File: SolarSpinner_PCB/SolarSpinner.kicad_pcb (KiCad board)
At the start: 2 copper layers, 50 x 40 mm, 21 parts, among them IC1 ATTINY85-P, P1 SOLAR, P10 HOLES, P2 SOLAR_V, P3 MOTOR, P4 ISP, P5 HEADER, P7 LOGO1, P8 LOGO2, Q1 Q_NPN_CBE

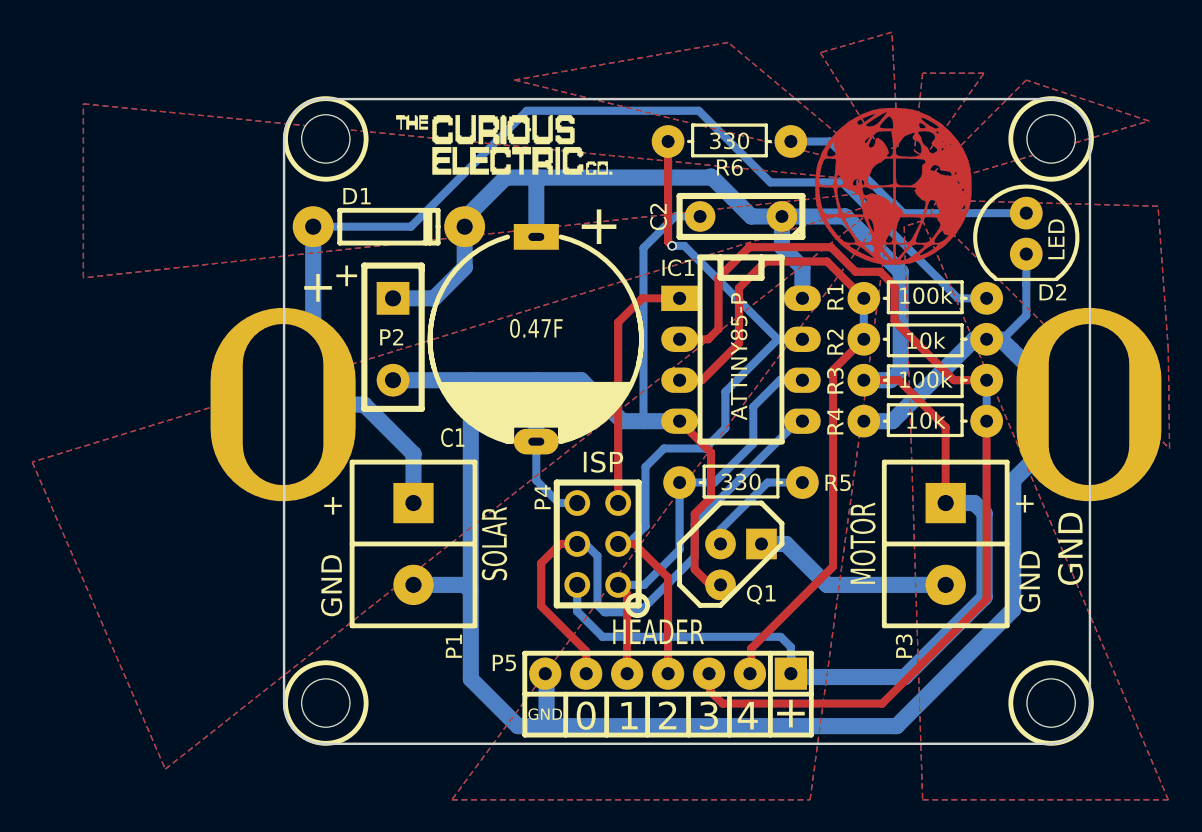
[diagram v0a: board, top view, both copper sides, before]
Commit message: Updated PCB. New Gerber
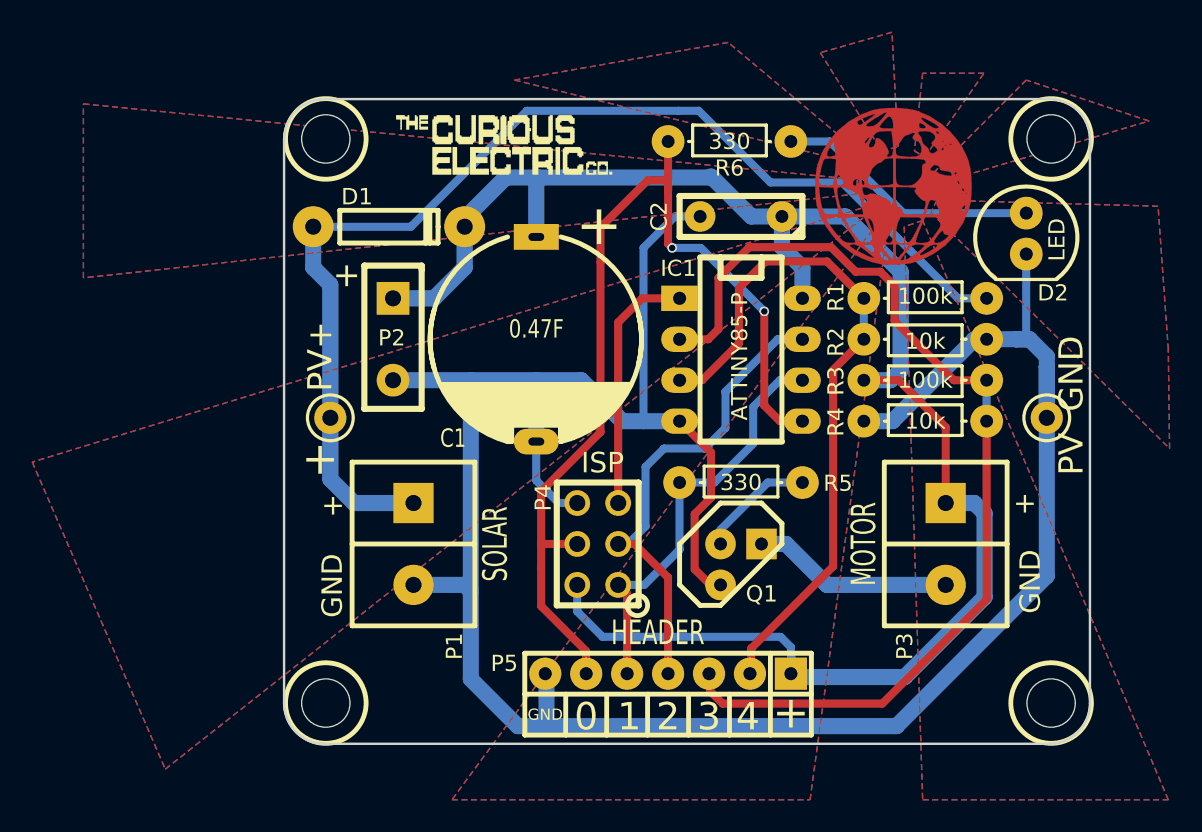
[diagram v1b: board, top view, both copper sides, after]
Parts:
- Q1: value Q_NPN_CBE -> BC547
- SC1: footprint REInnovationFootprint:PV_50x30mm -> REInnovationFootprint:PV_50x30mm_round
- moved SC1 1.07 mm to (149.9, 120.0)
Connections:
- R6 pad 1: Net-(IC1-Pad7) -> Net-(IC1-Pad5)
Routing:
- net Net-(IC1-Pad5): track 34.4 -> 62.4 mm, vias 0 -> 2
- net Net-(IC1-Pad7): track 46.8 -> 31.2 mm, vias 1 -> 0
- net GND: track 245.3 -> 241.8 mm
- net Net-(D1-Pad2): track 73.9 -> 71.5 mm
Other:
- net class Default: trace_width 0.5 -> 1
- board text added: "PV GND"
- board text added: "PV+"
- board text removed: "GND"
